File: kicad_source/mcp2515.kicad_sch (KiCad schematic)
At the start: 14 parts, among them CN4 GH_SM04B-GHS-TB, CN5 GH_SM04B-GHS-TB, U8 MCP2515, U9 SN65HVD232, Y1 16MHz

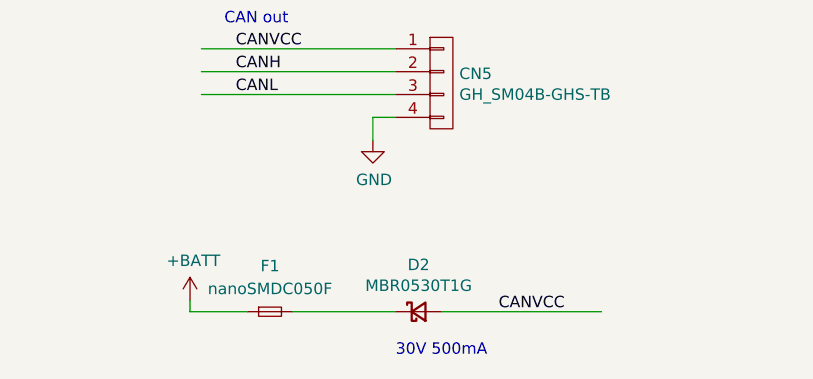
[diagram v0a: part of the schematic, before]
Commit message: reworked schematic
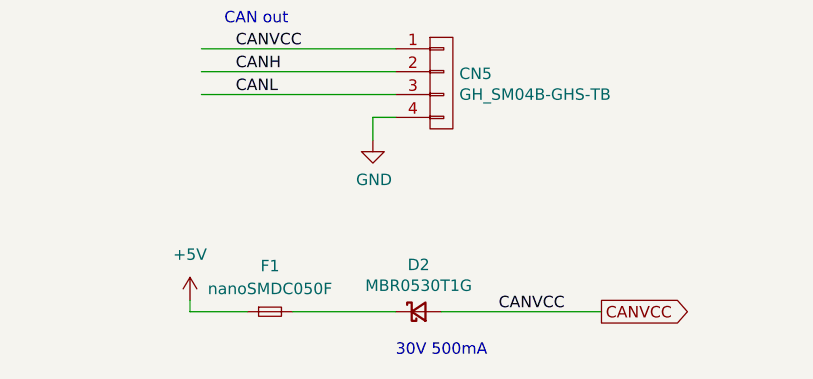
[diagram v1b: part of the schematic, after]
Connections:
- net +BATT renamed +5V
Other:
- title: OpenCyphalPicoBase -> OpenCyphalServoController12
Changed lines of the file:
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@@
   (paper "A4")
   (title_block
-    (title "OpenCyphalPicoBase")
-    (date "2022-06-09")
-    (rev "dev_0.1")
+    (title "OpenCyphalServoController12")
+    (date "2023-01-23")
+    (rev "0.1")
     (company "generationmake")
   )
@@
     (property "Referenzen zwischen Schaltplänen" "${INTERSHEET_REFS}" (id 0) (at 0 0 0)
       (effects (font (size 1.27 1.27)) hide)
+    )
+  )
+  (global_label "CANVCC" (shape output) (at 241.3 156.21 0) (fields_autoplaced)
+    (effects (font (size 1.27 1.27)) (justify left))
+    (property "Referenzen zwischen Schaltplänen" "${INTERSHEET_REFS}" (id 0) (at 250.9418 156.1306 0)
+      (effects (font (size 1.27 1.27)) (justify left) hide)
     )
   )
@@
     (pin "1")
   )
-  (symbol (lib_id "OpenCyphalPicoBase-rescue:+BATT-power-supply") (at 195.58 154.94 0) (unit 1)
-    (in_bom yes) (on_board yes)
-    (property "Reference" "#PWR038" (id 0) (at 195.58 158.75 0)
-      (effects (font (size 1.27 1.27)) hide)
-    )
-    (property "Value" "+BATT" (id 1) (at 195.961 150.5458 0))
-    (property "Footprint" "" (id 2) (at 195.58 154.94 0))
-    (property "Datasheet" "" (id 3) (at 195.58 154.94 0))
-    (pin "1")
-  )
   (symbol (lib_id "OpenCyphalPicoBase-rescue:GND-power-supply") (at 243.84 45.72 0) (unit 1)
     (in_bom yes) (on_board yes)
@@
     (pin "1")
   )
+  (symbol (lib_id "power:+5V") (at 195.58 154.94 0) (unit 1)
+    (in_bom yes) (on_board yes) (fields_autoplaced)
+    (property "Reference" "#PWR?" (id 0) (at 195.58 158.75 0)
+      (effects (font (size 1.27 1.27)) hide)
+    )
+    (property "Value" "+5V" (id 1) (at 195.58 149.86 0))
+    (property "Footprint" "" (id 2) (at 195.58 154.94 0)
+      (effects (font (size 1.27 1.27)) hide)
+    )
+    (property "Datasheet" "" (id 3) (at 195.58 154.94 0)
+      (effects (font (size 1.27 1.27)) hide)
+    )
+    (pin "1")
+  )
